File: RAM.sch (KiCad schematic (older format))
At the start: 13 parts, among them J9 RAM_CURRENT, U1 ATXMEGA128A1U-AU, U2 SN74AHC573PW, U3 IDT71V256SA

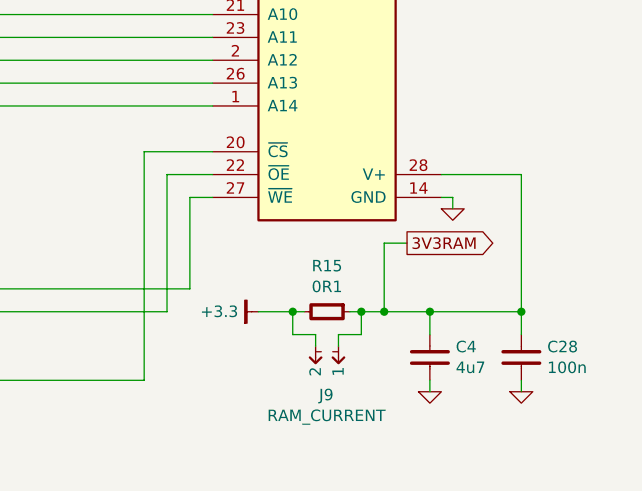
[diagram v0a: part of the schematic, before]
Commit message: Finished?
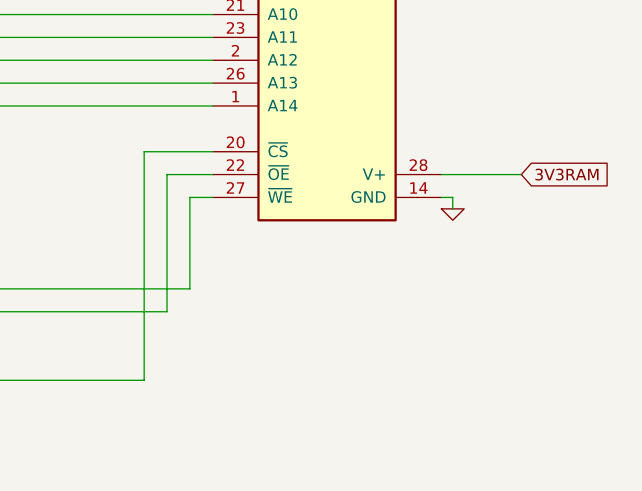
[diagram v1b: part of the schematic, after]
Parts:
- removed C28: 100n, IPC7351-Nominal:CAPC1005X55, symbol C-0402
- removed C4: 4u7, IPC7351-Nominal:CAPC1608X55, symbol C-0603
- removed J9: RAM_CURRENT, conn-100mil:CONN-100MIL-M-1x2, symbol CONN-100MIL-M-1x2
- removed R15: 0R1, IPC7351-Nominal:RESC1608X50, symbol R-0603
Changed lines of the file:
@@
 P 7100 5050
 AR Path="/56EF5511" Ref="#PWR?"  Part="1"
-AR Path="/56EF4451/56EF5511" Ref="#PWR?"  Part="1"
-F 0 "#PWR?" H 7100 5050 30  0001 C CNN
+AR Path="/56EF4451/56EF5511" Ref="#PWR21"  Part="1"
+F 0 "#PWR21" H 7100 5050 30  0001 C CNN
 F 1 "GND" H 7100 4980 30  0001 C CNN
 F 2 "" H 7100 5050 60  0000 C CNN
 F 3 "" H 7100 5050 60  0000 C CNN
 	1    7100 5050
-	1    0    0    -1
-$EndComp
-$Comp
-L C-0603 C?
-U 1 1 56EF5518
-P 7000 5700
-AR Path="/56EF5518" Ref="C?"  Part="1"
-AR Path="/56EF4451/56EF5518" Ref="C4"  Part="1"
-F 0 "C4" H 7113 5746 50  0000 L CNN
-F 1 "4u7" H 7113 5655 50  0000 L CNN
-F 2 "IPC7351-Nominal:CAPC1608X55" H 7000 5700 50  0001 C CNN
-F 3 "" H 6990 5675 60  0000 C CNN
-F 4 "CAP MLCC 4u7 10V ≥X5R 20% [0603]" H 7800 6250 60  0001 C CNN "BOM"
-	1    7000 5700
-	1    0    0    -1
-$EndComp
-$Comp
-L GND #PWR?
-U 1 1 56EF551F
-P 7000 5850
-AR Path="/56EF551F" Ref="#PWR?"  Part="1"
-AR Path="/56EF4451/56EF551F" Ref="#PWR?"  Part="1"
-F 0 "#PWR?" H 7000 5850 30  0001 C CNN
-F 1 "GND" H 7000 5780 30  0001 C CNN
-F 2 "" H 7000 5850 60  0000 C CNN
-F 3 "" H 7000 5850 60  0000 C CNN
-	1    7000 5850
-	1    0    0    -1
-$EndComp
-$Comp
-L C-0402 C?
-U 1 1 56EF5526
-P 7400 5700
-AR Path="/56EF5526" Ref="C?"  Part="1"
-AR Path="/56EF4451/56EF5526" Ref="C28"  Part="1"
-F 0 "C28" H 7513 5746 50  0000 L CNN
-F 1 "100n" H 7513 5655 50  0000 L CNN
-F 2 "IPC7351-Nominal:CAPC1005X55" H 7400 5700 50  0001 C CNN
-F 3 "" H 7390 5675 60  0000 C CNN
-F 4 "CAP MLCC 100n ≥X5R 10V 20% [0402]" H 8200 6250 60  0001 C CNN "BOM"
-	1    7400 5700
-	1    0    0    -1
-$EndComp
-$Comp
-L GND #PWR?
-U 1 1 56EF552D
-P 7400 5850
-AR Path="/56EF552D" Ref="#PWR?"  Part="1"
-AR Path="/56EF4451/56EF552D" Ref="#PWR?"  Part="1"
-F 0 "#PWR?" H 7400 5850 30  0001 C CNN
-F 1 "GND" H 7400 5780 30  0001 C CNN
-F 2 "" H 7400 5850 60  0000 C CNN
-F 3 "" H 7400 5850 60  0000 C CNN
-	1    7400 5850
 	1    0    0    -1
 $EndComp
@@
 P 5000 3000
 AR Path="/56EF553D" Ref="#PWR?"  Part="1"
-AR Path="/56EF4451/56EF553D" Ref="#PWR?"  Part="1"
-F 0 "#PWR?" H 5000 3000 30  0001 C CNN
+AR Path="/56EF4451/56EF553D" Ref="#PWR20"  Part="1"
+F 0 "#PWR20" H 5000 3000 30  0001 C CNN
 F 1 "GND" H 5000 2930 30  0001 C CNN
 F 2 "" H 5000 3000 60  0000 C CNN
@@
 	7100 5000 7050 5000
 Wire Wire Line
-	7000 5500 7000 5600
-Wire Wire Line
-	7000 5850 7000 5800
-Wire Wire Line
-	7400 4900 7400 5600
-Wire Wire Line
-	7400 5850 7400 5800
-Wire Wire Line
 	6050 3200 5750 3200
 Wire Wire Line
@@
 Wire Wire Line
 	3050 4700 3100 4700
-Wire Wire Line
-	6650 5500 7400 5500
-$Comp
-L +3.3 #PWR?
-U 1 1 56EF5658
-P 6250 5500
-AR Path="/56EF5658" Ref="#PWR?"  Part="1"
-AR Path="/56EF4451/56EF5658" Ref="#PWR?"  Part="1"
-F 0 "#PWR?" H 6250 5550 30  0001 C CNN
-F 1 "+3.3" V 6250 5588 50  0000 L CNN
-F 2 "" H 6250 5500 60  0000 C CNN
-F 3 "" H 6250 5500 60  0000 C CNN
-	1    6250 5500
-	0    -1   -1   0
-$EndComp
-$Comp
-L R-0603 R?
-U 1 1 56EF565F
-P 6550 5500
-AR Path="/56EF565F" Ref="R?"  Part="1"
-AR Path="/56EF4451/56EF565F" Ref="R15"  Part="1"
-F 0 "R15" V 6350 5500 50  0000 C CNN
-F 1 "0R1" V 6441 5500 50  0000 C CNN
-F 2 "IPC7351-Nominal:RESC1608X50" H 6550 5500 50  0001 C CNN
-F 3 "" H 6550 5550 60  0000 C CNN
-F 4 "RES SMD 0R1 1% [0603]" H 7300 6050 60  0001 C CNN "BOM"
-	1    6550 5500
-	0    1    1    0
-$EndComp
-Wire Wire Line
-	6250 5500 6450 5500
-$Comp
-L CONN-100MIL-M-1x2 J?
-U 1 1 56EF5668
-P 6600 5700
-AR Path="/56EF5668" Ref="J?"  Part="1"
-AR Path="/56EF4451/56EF5668" Ref="J9"  Part="1"
-F 0 "J9" V 6764 5647 50  0000 C CNN
-F 1 "RAM_CURRENT" V 6855 5647 50  0000 C CNN
-F 2 "conn-100mil:CONN-100MIL-M-1x2" H 6600 5700 50  0001 C CNN
-F 3 "" H 6600 5700 50  0000 C CNN
-F 4 "DIST DIGIKEY 3M9447-ND" H 6600 5700 60  0001 C CNN "BOM"
-	1    6600 5700
-	0    1    1    0
-$EndComp
-Wire Wire Line
-	6500 5650 6500 5600
-Wire Wire Line
-	6500 5600 6400 5600
-Wire Wire Line
-	6400 5600 6400 5500
-Connection ~ 6400 5500
-Wire Wire Line
-	6600 5650 6600 5600
-Wire Wire Line
-	6600 5600 6700 5600
-Wire Wire Line
-	6700 5600 6700 5500
-Connection ~ 6700 5500
-Text GLabel 6900 5200 2    50   Output ~ 0
+Text GLabel 7400 4900 2    50   Input ~ 0
 3V3RAM
-Wire Wire Line
-	6900 5200 6800 5200
-Wire Wire Line
-	6800 5200 6800 5500
-Connection ~ 6800 5500
-Connection ~ 7000 5500
-Connection ~ 7400 5500
 $Comp
 L TESTPOINT TP?
@@
 P 3700 3350
 AR Path="/56EF5685" Ref="#PWR?"  Part="1"
-AR Path="/56EF4451/56EF5685" Ref="#PWR?"  Part="1"
-F 0 "#PWR?" H 3700 3350 30  0001 C CNN
+AR Path="/56EF4451/56EF5685" Ref="#PWR19"  Part="1"
+F 0 "#PWR19" H 3700 3350 30  0001 C CNN
 F 1 "GND" H 3700 3280 30  0001 C CNN
 F 2 "" H 3700 3350 60  0000 C CNN
